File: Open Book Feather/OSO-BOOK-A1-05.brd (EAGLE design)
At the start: 77.5 x 112.3 mm, 133 parts, among them J1 SJ-43514-SMT, J2 10118193-0001LF, Q1 DMG341, Q2 IRLML0100, SW1 SPDT_SWITCH, U1 AP2112-3.3, U2 MCP73831T-2ACI/OT, U3 ATSAMD51J64-TQFP(10X10), U4 GD25Q16C (or GD25Q32C), U5 74AC165D, U6 GD25Q16C (or GD25Q32C), U7 MAX4468EKAT, X1 JSTPH, X2 2x5 0.05" SWD

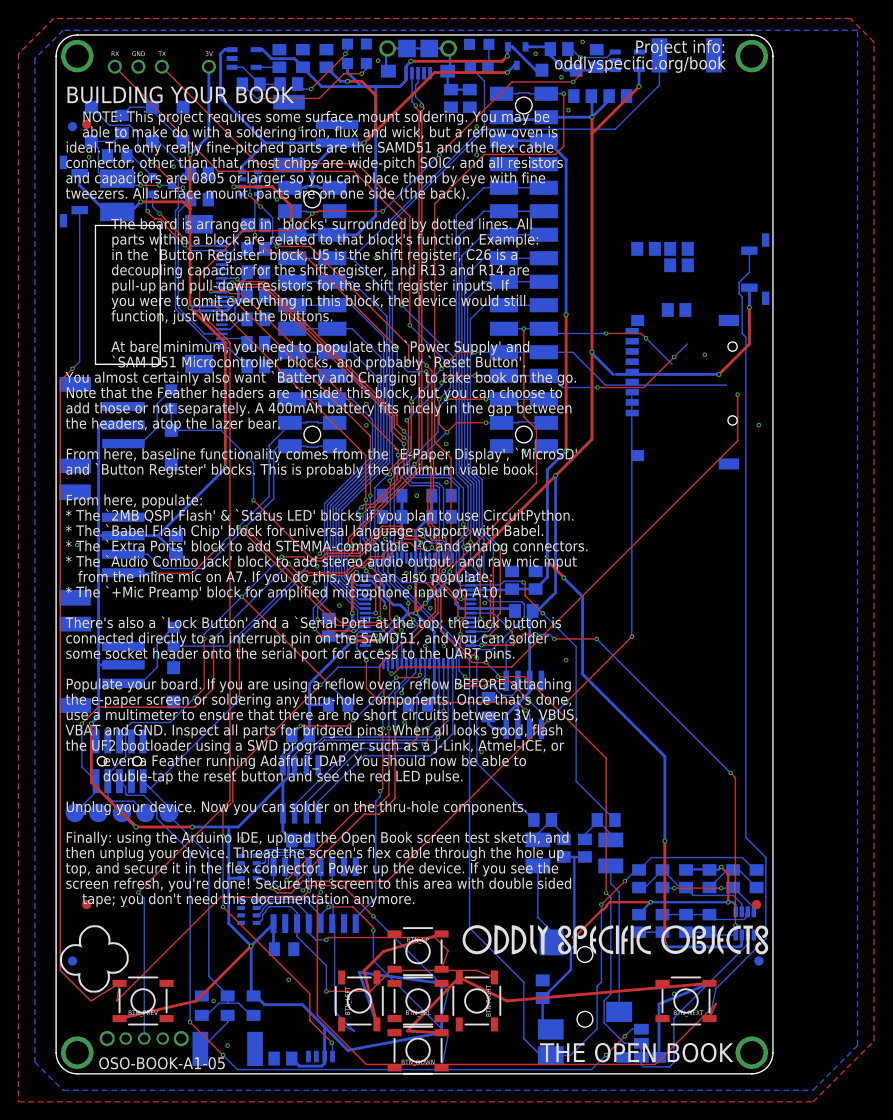
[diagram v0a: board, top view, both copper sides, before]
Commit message: Revert "Buttons & SD card change"
This reverts commit 564ec3b5048e0d7899cd32f6cb14d9a07736022d.
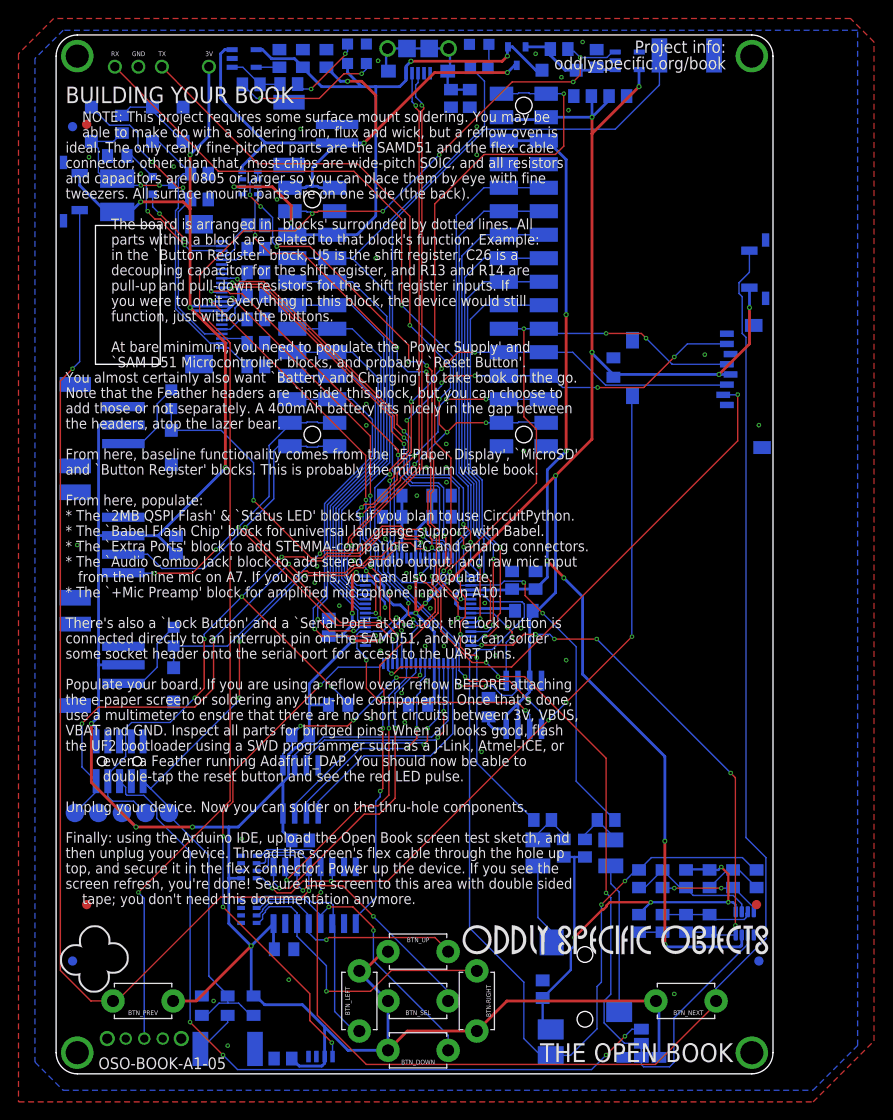
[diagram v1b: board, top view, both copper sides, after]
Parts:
- removed C37: 10uF, rcl:C0805
- removed R28, R29, R30: 10K, rcl:R0805
- removed SD_CARD: MICRO_SD_CARD_, dronecz:TFP09-2--12B
- added C25: 10uF, microbuilder:0805_10MGAP
- added MICROSD: MICROSD, adafruit:MICROSD
- BTN-RIGHT, BTN_DOWN, BTN_LEFT, BTN_NEXT, BTN_PREV, BTN_SEL, BTN_UP: value TACTILE_SWITCHE_5X5_MICRO_ -> (none); device dronecz:TACTILE_SWITCH_5X5_MICRO -> adafruit:TACT_PANA-EVQ
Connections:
- net +3V3: now also BTN-RIGHT.P$2, BTN_DOWN.P$2, BTN_LEFT.P$2, BTN_NEXT.P$2, BTN_PREV.P$2, BTN_SEL.P$2, BTN_UP.P$2, C25.1, MICROSD.4; no longer BTN-RIGHT.3, BTN_DOWN.3, BTN_LEFT.3, BTN_NEXT.3, BTN_PREV.3, BTN_SEL.3, BTN_UP.3, C37.1, R28.2, R29.2, R30.2, SD_CARD.VCC
- net BUTTON0: now also BTN_LEFT.P$1; no longer BTN_LEFT.1
- net BUTTON1: now also BTN_DOWN.P$1; no longer BTN_DOWN.1
- net BUTTON2: now also BTN_UP.P$1; no longer BTN_UP.1
- net BUTTON3: now also BTN-RIGHT.P$1; no longer BTN-RIGHT.1
- net BUTTON4: now also BTN_SEL.P$1; no longer BTN_SEL.1
- net BUTTON5: now also BTN_PREV.P$1; no longer BTN_PREV.1
- net BUTTON6: now also BTN_NEXT.P$1; no longer BTN_NEXT.1, BTN_NEXT.2
- net BUTTON7: now also MICROSD.CD2; no longer SD_CARD.CD
- net GND: now also C25.2, MICROSD.6, MICROSD.MT1, MICROSD.MT2; no longer C37.2, SD_CARD.GND, SD_CARD.GND@1, SD_CARD.GND@2, SD_CARD.GND@3, SD_CARD.VSS
- net MISO: now also MICROSD.7; no longer R30.1, SD_CARD.DAT0
- net MOSI: now also MICROSD.3; no longer R28.1, SD_CARD.CMD
- net SCK: now also MICROSD.5; no longer R29.1, SD_CARD.CLK
- net SDCS: now also MICROSD.2; no longer SD_CARD.CD/DAT3
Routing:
- net +3V3: track 558.1 -> 512.4 mm
- net SCK: track 92.8 -> 98.8 mm
- net MISO: track 77.0 -> 81.3 mm
- net BUTTON6: track 161.4 -> 158.0 mm
- net BUTTON5: track 129.1 -> 126.3 mm
- net BUTTON2: track 27.0 -> 25.0 mm
- net BUTTON3: track 34.8 -> 32.7 mm
- net BUTTON4: track 33.1 -> 31.2 mm
- net BUTTON1: track 34.5 -> 32.6 mm
- net SDCS: track 54.1 -> 55.7 mm
- net BUTTON0: track 25.0 -> 24.0 mm
